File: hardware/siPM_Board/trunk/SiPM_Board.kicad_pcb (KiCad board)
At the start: 4 copper layers, 50.7 x 50.7 mm, 17 parts, among them J1 Conn_02x34_Odd_Even, J2 Conn_02x34_Odd_Even, U1 LM94021, U2 S14161-6050HS-04, U3 S14161-6050HS-04, U4 S14161-6050HS-04, U5 S14161-6050HS-04

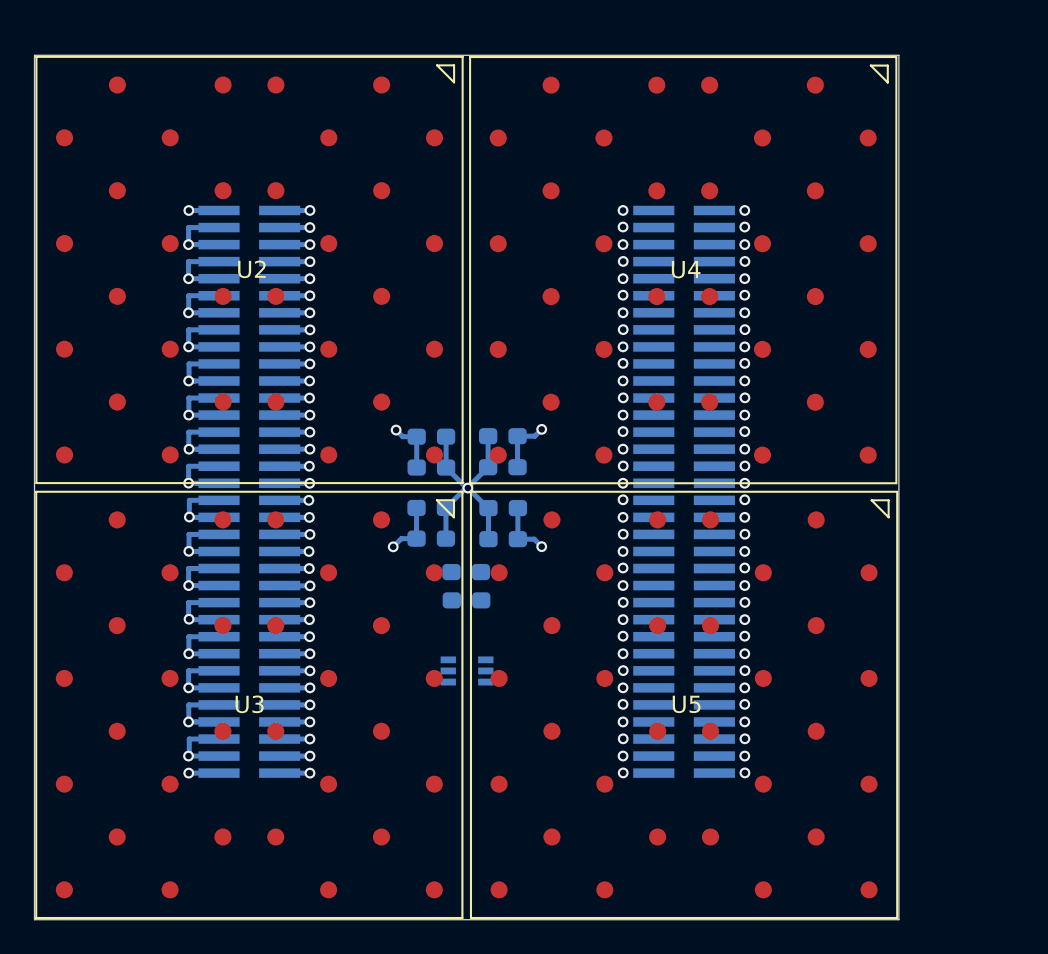
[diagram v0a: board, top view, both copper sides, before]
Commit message: Tracing incomplete
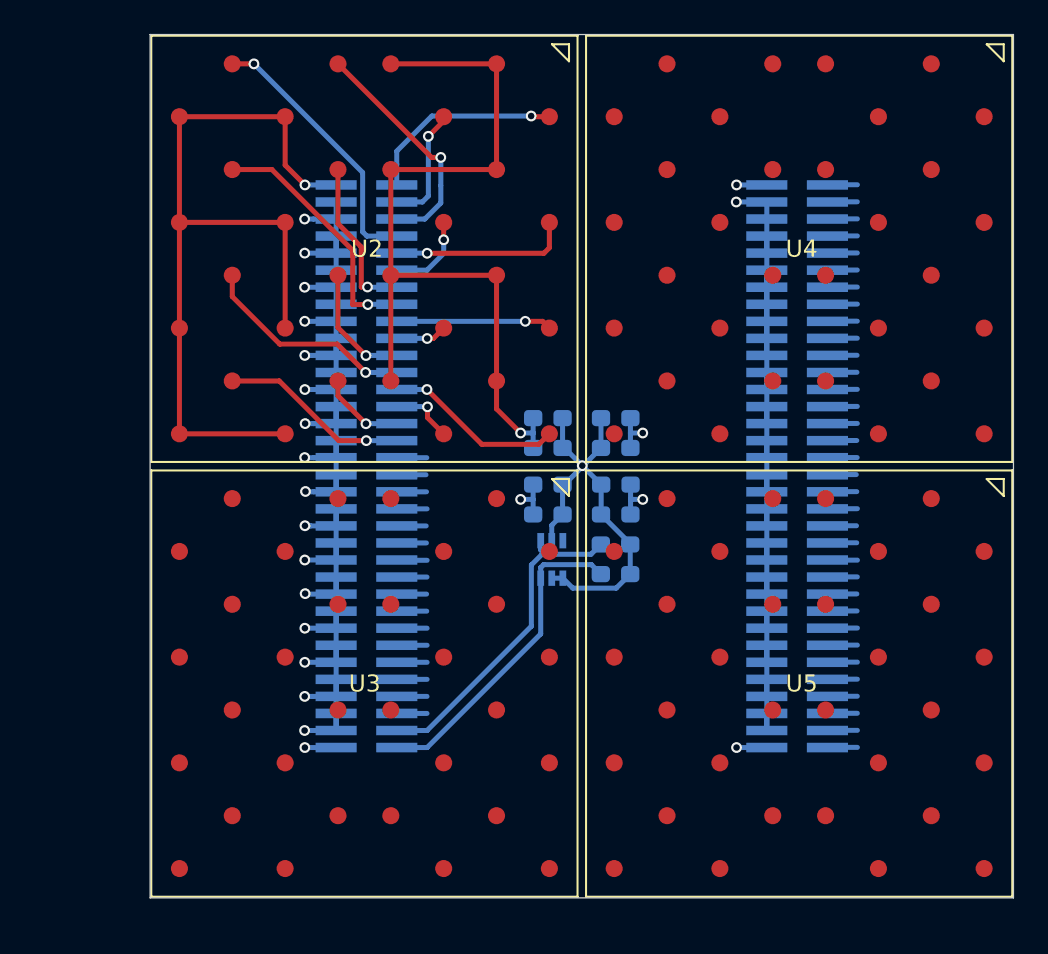
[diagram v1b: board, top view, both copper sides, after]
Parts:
- moved C9 8.91 mm to (152.0, 104.6)
- moved C10 8.87 mm to (152.0, 106.3)
- moved U1 8.21 mm to (148.2, 105.5), turned to 90 degrees
- moved J1 7.03 mm to (137.4, 100.0)
- moved C4 6.99 mm to (148.0, 102.8)
- moved C3 6.98 mm to (148.0, 101.1)
- moved C1 6.93 mm to (148.0, 98.9)
- moved C2 6.92 mm to (148.0, 97.2)
- moved U4 6.91 mm to (162.8, 87.2)
- moved U3 6.86 mm to (137.2, 112.8)
- moved U5 6.86 mm to (162.8, 112.8)
- moved U2 6.85 mm to (137.2, 87.2)
- moved J2 6.80 mm to (162.6, 100.0)
- moved C7 6.76 mm to (152.0, 102.8)
- moved C8 6.75 mm to (152.0, 101.1)
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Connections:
- J1 pad 67: /BIAS2 -> /OUT
- J1 pad 68: /OUT -> /BIAS2
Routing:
- net /BIAS1: track 4.95 -> 99.2 mm
- net GND: track 87.1 -> 149.2 mm, vias 17 -> 18
- net /VDD: track 1.78 -> 19.5 mm, vias 1 -> 0
- net /OUT: track 1.77 -> 18.9 mm, vias 1 -> 0
- net Net-(J1-Pad7): track 1.78 -> 15.9 mm
- net Net-(J1-Pad15): track 1.78 -> 14.8 mm
- net Net-(J1-Pad5): track 1.78 -> 13.9 mm
- net Net-(J1-Pad23): track 1.75 -> 12.7 mm
- net Net-(J1-Pad1): track 2.46 -> 12.5 mm
- net Net-(J1-Pad31): track 1.74 -> 11.1 mm
- net Net-(J1-Pad9): track 1.77 -> 10.6 mm
- net Net-(J1-Pad25): track 1.77 -> 10.5 mm
- net Net-(J1-Pad13): track 1.77 -> 9.54 mm
- net Net-(J1-Pad17): track 1.77 -> 9.12 mm
- net Net-(J1-Pad21): track 1.76 -> 7.20 mm
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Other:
- board size 50.7 x 50.7 mm -> 50.6 x 50.6 mm
